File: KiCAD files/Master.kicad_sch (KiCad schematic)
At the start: 24 parts, among them SW1 EG1271A, SW2 EG1271A, SW3 EG1271A, SW4 EG1271A, U4 NUCLEO64-F446RE

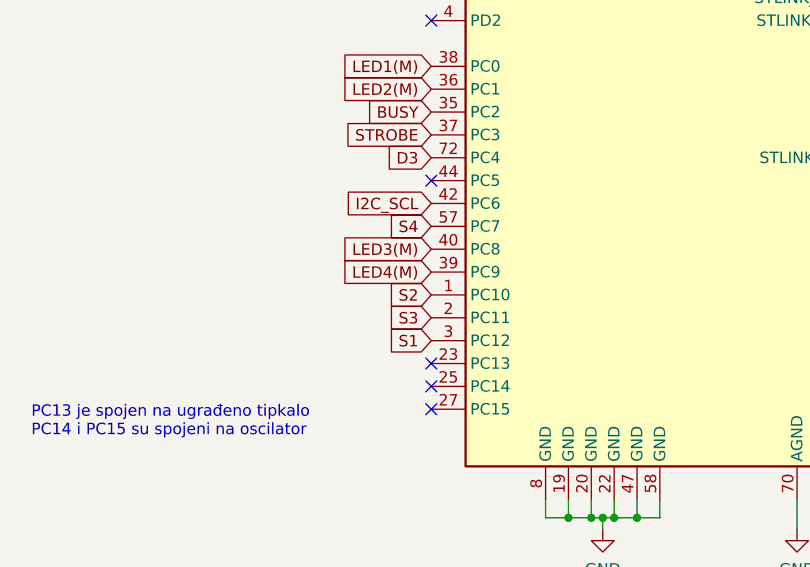
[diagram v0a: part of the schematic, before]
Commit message: update
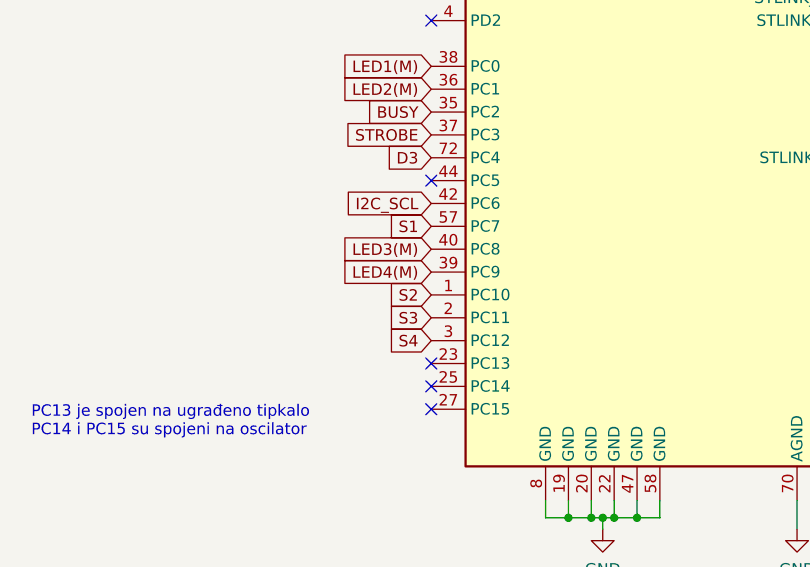
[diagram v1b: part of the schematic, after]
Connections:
- net S1: now also U4.57 (PC7); no longer U4.3 (PC12)
- net S4: now also U4.3 (PC12); no longer U4.57 (PC7)
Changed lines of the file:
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@@
     )
   )
-  (global_label "S4" (shape input) (at 113.665 111.76 180) (fields_autoplaced)
+  (global_label "S4" (shape input) (at 113.665 124.46 180) (fields_autoplaced)
     (effects (font (size 1.27 1.27)) (justify right))
-    (property "Intersheetrefs" "${INTERSHEET_REFS}" (at 108.2608 111.76 0)
+    (property "Intersheetrefs" "${INTERSHEET_REFS}" (at 108.2608 124.46 0)
       (effects (font (size 1.27 1.27)) (justify right) hide)
     )
@@
     )
   )
-  (global_label "S1" (shape input) (at 113.665 124.46 180) (fields_autoplaced)
+  (global_label "S1" (shape input) (at 113.665 111.76 180) (fields_autoplaced)
     (effects (font (size 1.27 1.27)) (justify right))
-    (property "Intersheetrefs" "${INTERSHEET_REFS}" (at 108.2608 124.46 0)
+    (property "Intersheetrefs" "${INTERSHEET_REFS}" (at 108.2608 111.76 0)
       (effects (font (size 1.27 1.27)) (justify right) hide)
     )

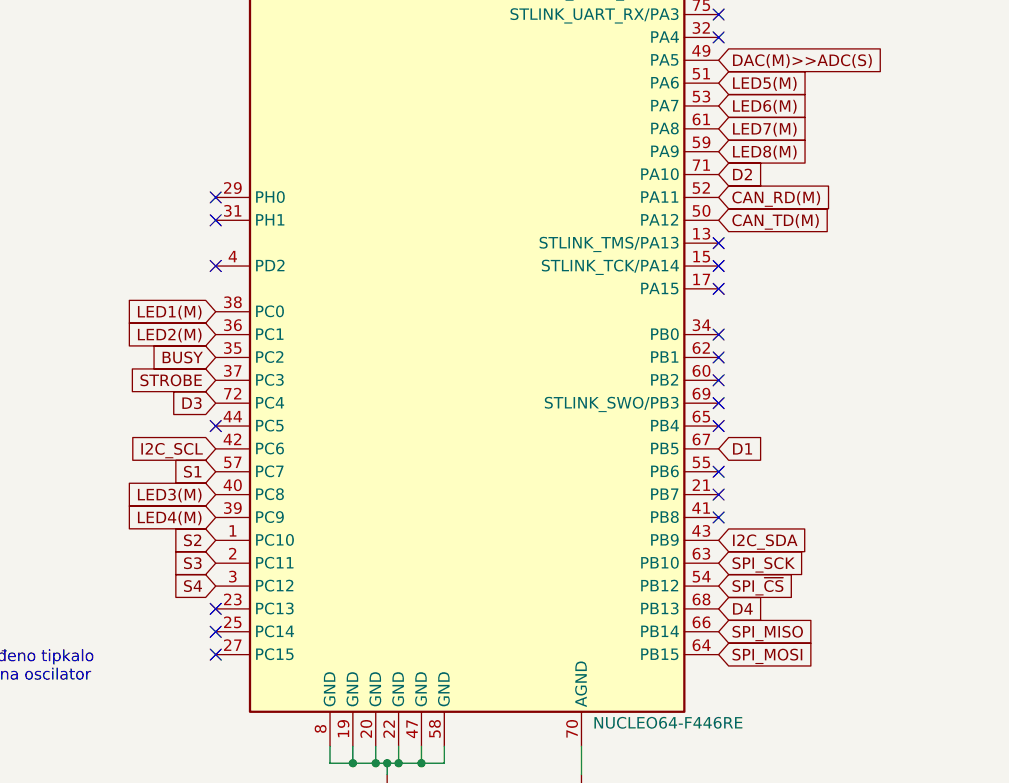
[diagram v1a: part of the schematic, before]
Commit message: update
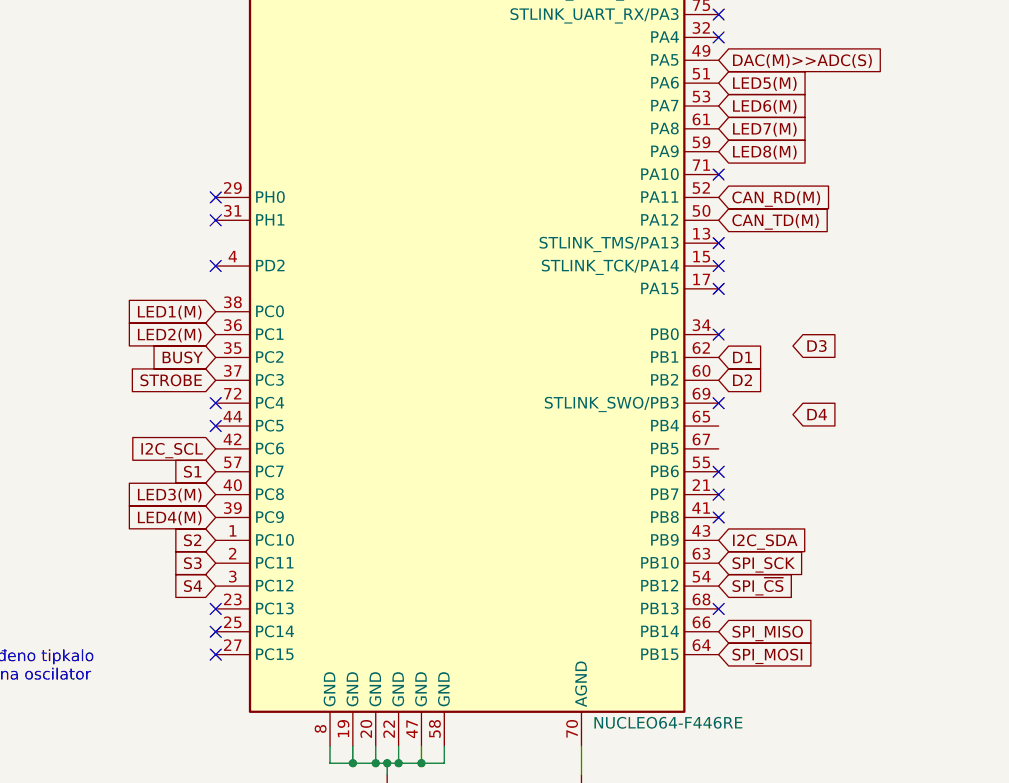
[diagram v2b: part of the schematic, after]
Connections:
- net D1: now also U4.62 (PB1); no longer U4.67 (PB5)
- net D2: now also U4.60 (PB2); no longer U4.71 (PA10)
- net D3: no longer U4.72 (PC4)
- net D4: no longer U4.68 (PB13)
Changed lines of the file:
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@@
   )
   (no_connect (at 169.545 111.76))
-  (no_connect (at 169.545 106.68))
   (no_connect (at 57.785 136.525))
   (no_connect (at 113.665 53.34))
@@
   (no_connect (at 57.785 147.32))
   (no_connect (at 113.665 55.88))
+  (no_connect (at 169.545 78.74))
   (no_connect (at 113.665 81.28))
   (no_connect (at 169.545 104.14))
   (no_connect (at 139.065 40.64))
   (no_connect (at 169.545 114.3))
+  (no_connect (at 113.665 104.14))
   (no_connect (at 58.42 125.73))
   (no_connect (at 169.545 60.96))
@@
   (no_connect (at 144.145 40.64))
   (no_connect (at 131.445 40.64))
-  (no_connect (at 169.545 101.6))
   (no_connect (at 133.985 40.64))
   (no_connect (at 169.545 58.42))
@@
   (no_connect (at 128.905 40.64))
   (no_connect (at 113.665 88.9))
-  (no_connect (at 169.545 99.06))
   (no_connect (at 169.545 96.52))
   (no_connect (at 113.665 132.08))
+  (no_connect (at 169.545 127))
   (no_connect (at 126.365 40.64))
   (no_connect (at 169.545 86.36))
@@
     )
   )
-  (global_label "D4" (shape input) (at 169.545 127 0) (fields_autoplaced)
-    (effects (font (size 1.27 1.27)) (justify left))
-    (property "Intersheetrefs" "${INTERSHEET_REFS}" (at 175.0097 127 0)
+  (global_label "D4" (shape input) (at 177.8 105.41 0) (fields_autoplaced)
+    (effects (font (size 1.27 1.27)) (justify left))
+    (property "Intersheetrefs" "${INTERSHEET_REFS}" (at 183.2647 105.41 0)
       (effects (font (size 1.27 1.27)) (justify left) hide)
     )
@@
     )
   )
-  (global_label "D2" (shape input) (at 169.545 78.74 0) (fields_autoplaced)
-    (effects (font (size 1.27 1.27)) (justify left))
-    (property "Intersheetrefs" "${INTERSHEET_REFS}" (at 175.0097 78.74 0)
+  (global_label "D2" (shape input) (at 169.545 101.6 0) (fields_autoplaced)
+    (effects (font (size 1.27 1.27)) (justify left))
+    (property "Intersheetrefs" "${INTERSHEET_REFS}" (at 175.0097 101.6 0)
       (effects (font (size 1.27 1.27)) (justify left) hide)
     )
@@
     )
   )
-  (global_label "D3" (shape input) (at 113.665 104.14 180) (fields_autoplaced)
-    (effects (font (size 1.27 1.27)) (justify right))
-    (property "Intersheetrefs" "${INTERSHEET_REFS}" (at 108.2003 104.14 0)
-      (effects (font (size 1.27 1.27)) (justify right) hide)
+  (global_label "D3" (shape input) (at 177.8 97.79 0) (fields_autoplaced)
+    (effects (font (size 1.27 1.27)) (justify left))
+    (property "Intersheetrefs" "${INTERSHEET_REFS}" (at 183.2647 97.79 0)
+      (effects (font (size 1.27 1.27)) (justify left) hide)
     )
   )
@@
     )
   )
-  (global_label "D1" (shape input) (at 169.545 109.22 0) (fields_autoplaced)
-    (effects (font (size 1.27 1.27)) (justify left))
-    (property "Intersheetrefs" "${INTERSHEET_REFS}" (at 175.0097 109.22 0)
-      (effects (font (size 1.27 1.27)) (justify left) hide)
-    )
+  (global_label "D1" (shape input) (at 169.545 99.06 0) (fields_autoplaced)
+    (effects (font (size 1.27 1.27)) (justify left))
+    (property "Intersheetrefs" "${INTERSHEET_REFS}" (at 175.0097 99.06 0)
+      (effects (font (size 1.27 1.27)) (justify left) hide)
+    )

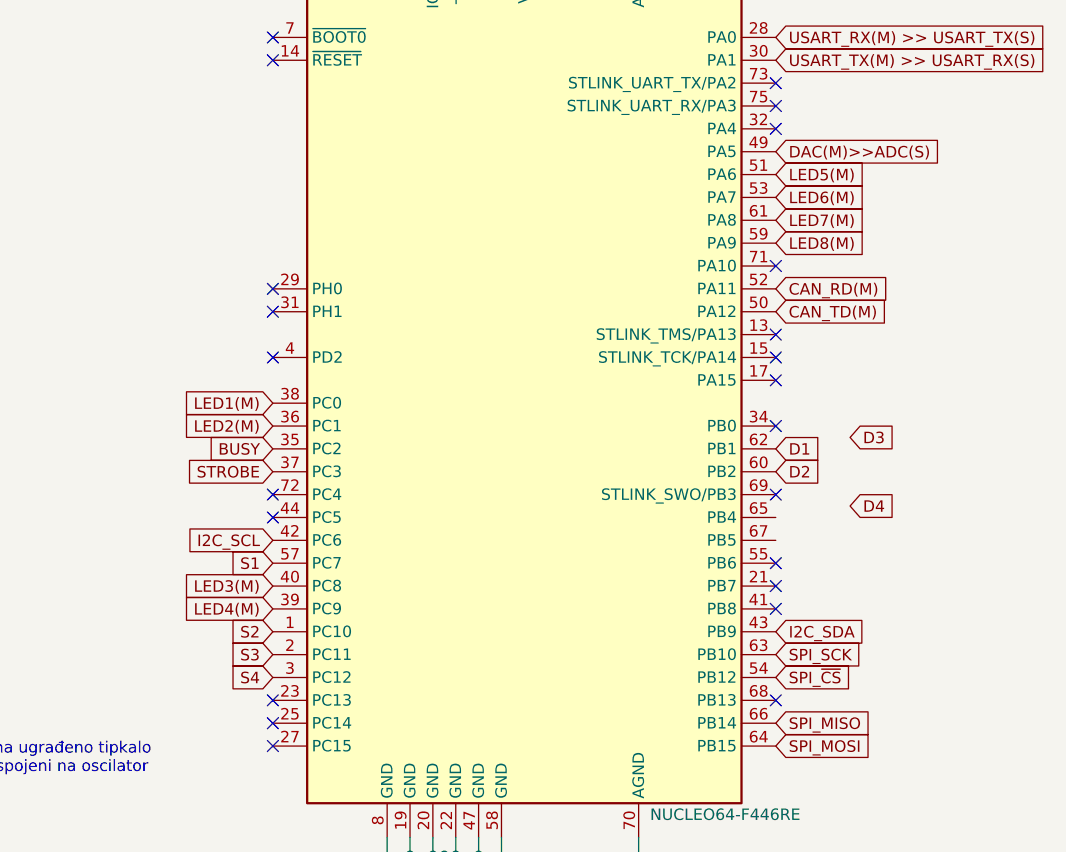
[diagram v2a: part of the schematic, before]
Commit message: update
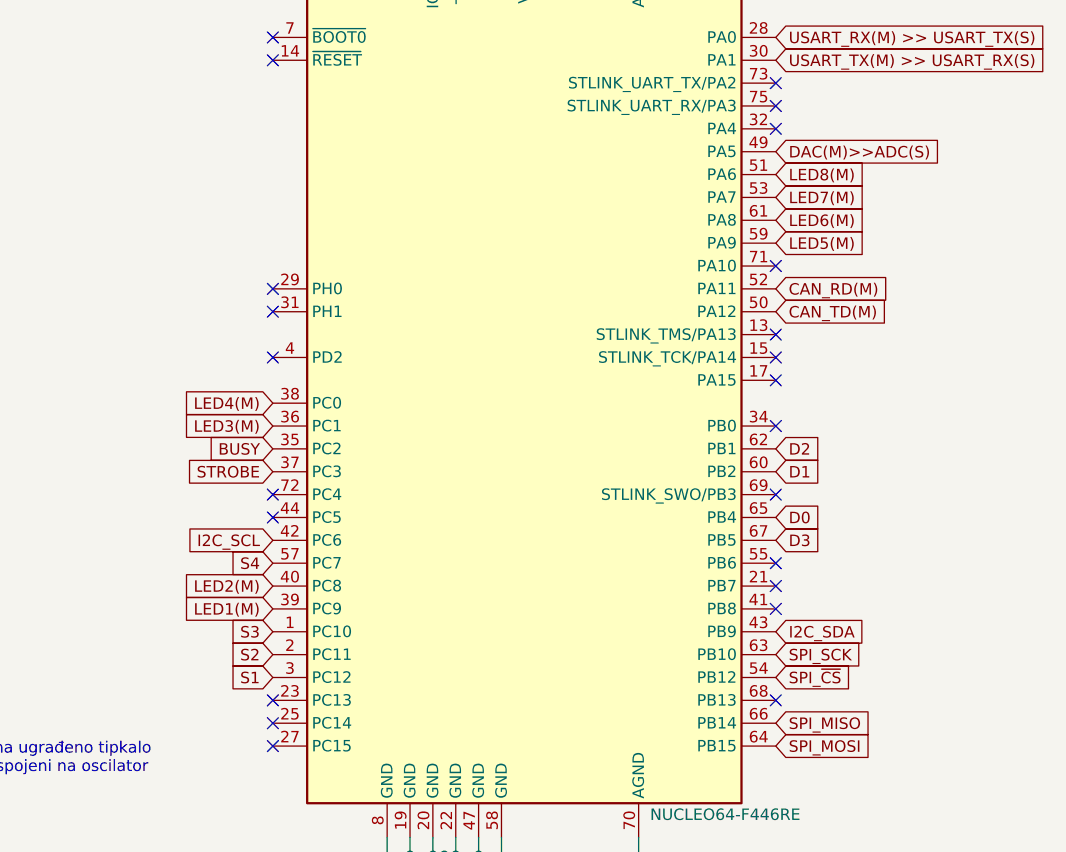
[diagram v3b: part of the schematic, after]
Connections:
- net D1: now also U4.60 (PB2); no longer U4.62 (PB1)
- net D2: now also U4.62 (PB1); no longer U4.60 (PB2)
- net D3: now also U4.67 (PB5)
- net LED1(M): now also U4.39 (PC9); no longer U4.38 (PC0)
- net LED2(M): now also U4.40 (PC8); no longer U4.36 (PC1)
- net LED3(M): now also U4.36 (PC1); no longer U4.40 (PC8)
- net LED4(M): now also U4.38 (PC0); no longer U4.39 (PC9)
- net LED5(M): now also U4.59 (PA9); no longer U4.51 (PA6)
- net LED6(M): now also U4.61 (PA8); no longer U4.53 (PA7)
- net LED7(M): now also U4.53 (PA7); no longer U4.61 (PA8)
- net LED8(M): now also U4.51 (PA6); no longer U4.59 (PA9)
- net S1: now also U4.3 (PC12); no longer U4.57 (PC7)
- net S2: now also U4.2 (PC11); no longer U4.1 (PC10)
- net S3: now also U4.1 (PC10); no longer U4.2 (PC11)
- net S4: now also U4.57 (PC7); no longer U4.3 (PC12)
- net D0: now reaches U4.65 (PB4)
